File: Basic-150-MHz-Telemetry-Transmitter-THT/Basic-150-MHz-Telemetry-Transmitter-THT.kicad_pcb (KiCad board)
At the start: 2 copper layers, 33.8 x 21.8 mm, 11 parts, among them J1 input/output, J2 Antenna, Q1 2N3904, Y1 Crystal_GND3

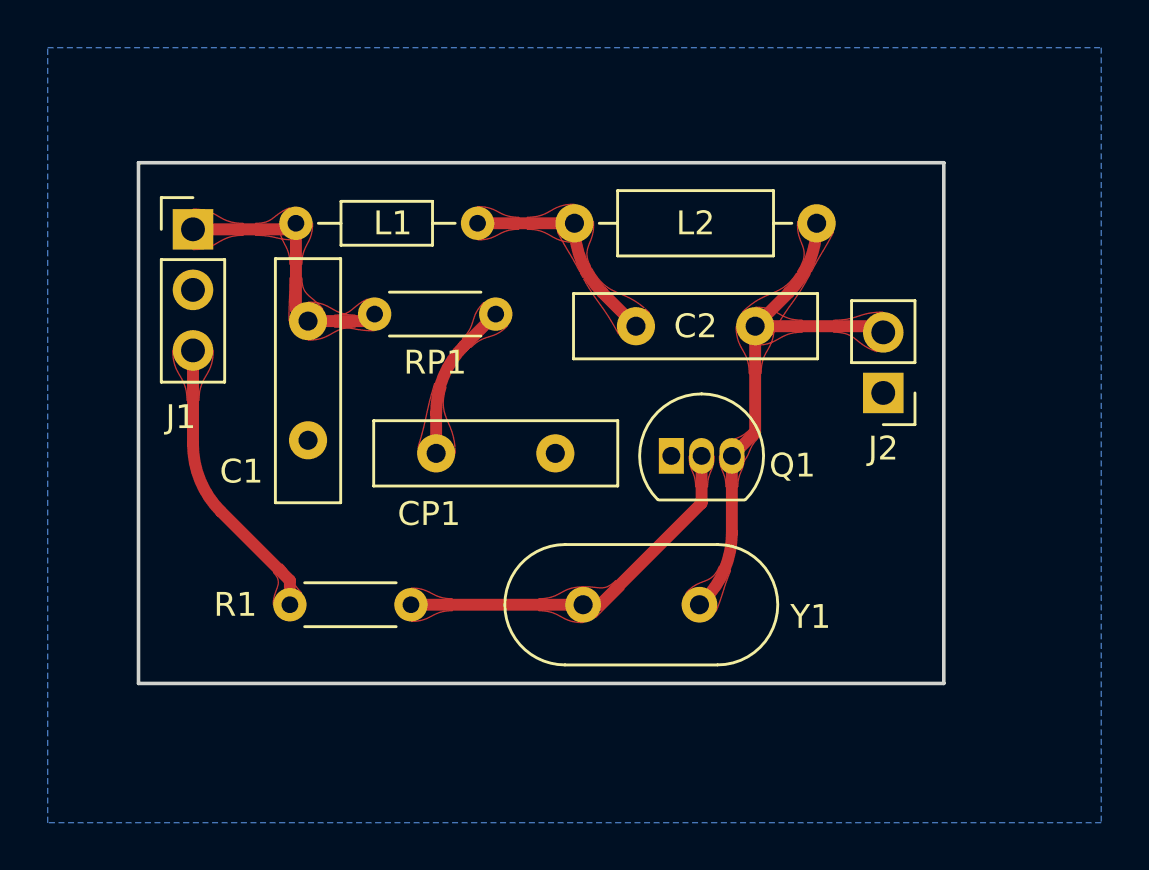
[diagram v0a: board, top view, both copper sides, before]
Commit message: h
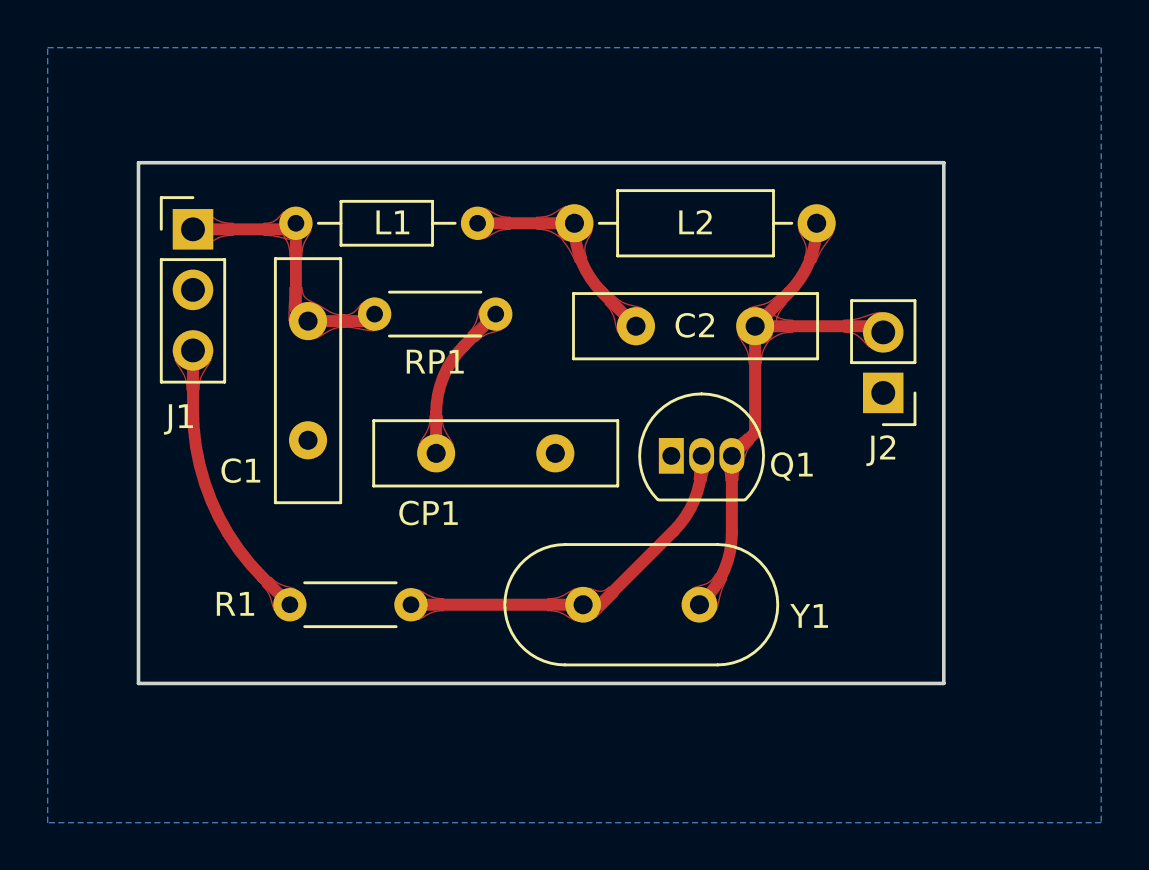
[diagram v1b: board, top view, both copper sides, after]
